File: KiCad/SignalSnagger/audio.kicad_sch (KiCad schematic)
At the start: 35 parts, among them J301 AudioJack4, U301 LM386, U302 LT6231

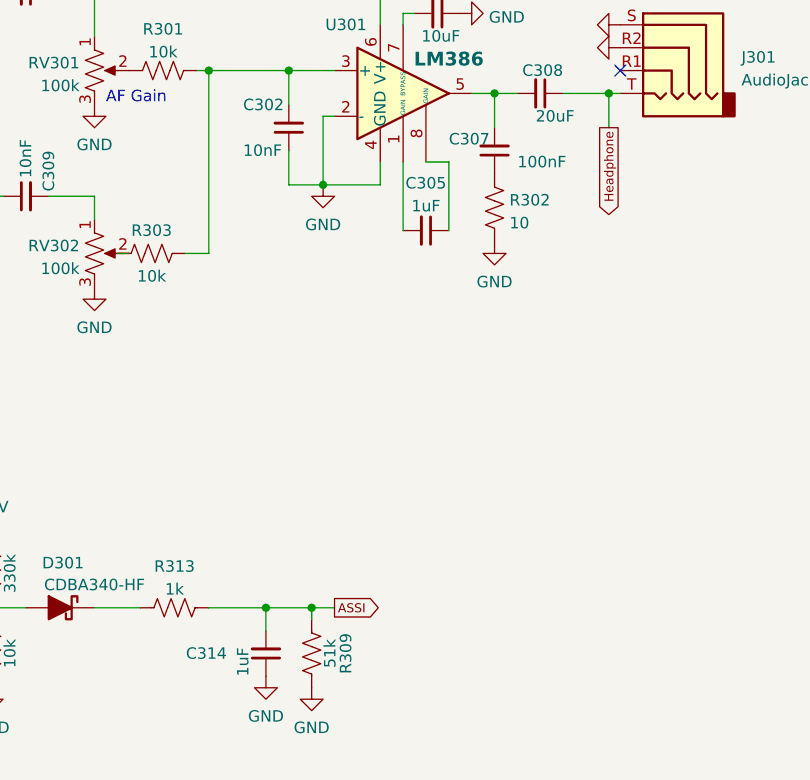
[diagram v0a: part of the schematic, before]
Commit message: Ver 0.22
o Schematic updates
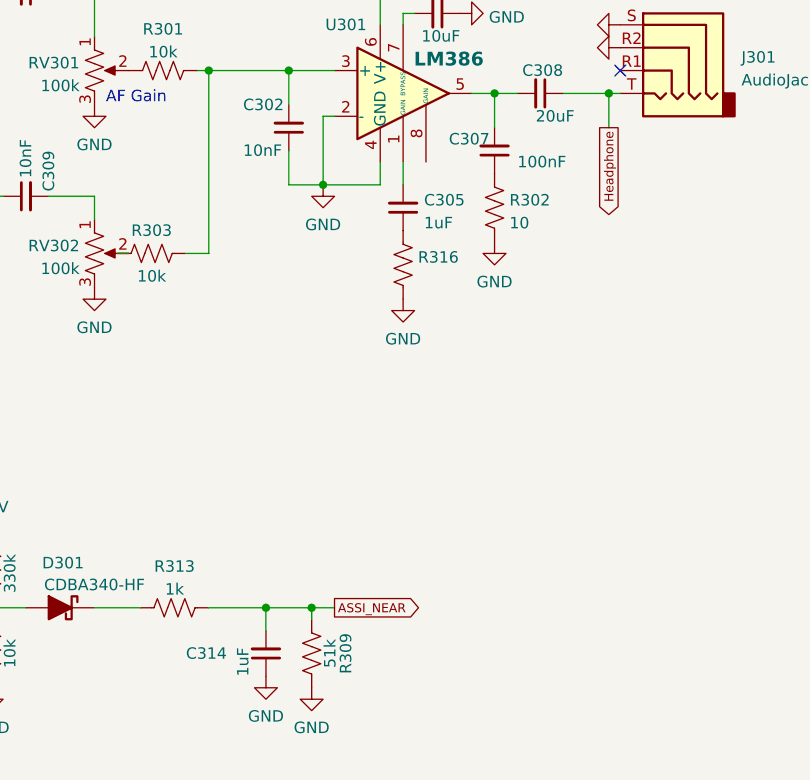
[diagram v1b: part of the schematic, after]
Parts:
- added R316: (no value), symbol Device:R_US
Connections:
- net GND: now also R316.2
- net at U301.8 (GAIN): no longer C305.1
- net ASSI renamed ASSI_NEAR
- new net: C305.1, R316.1
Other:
- moved on the sheet: C305
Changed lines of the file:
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@@
   (title_block
     (title "SignalSnagger")
-    (date "2023-12-19")
-    (rev "0.21")
+    (date "2024-02-01")
+    (rev "0.22")
   )
   (junction (at 66.04 128.27) (diameter 0) (color 0 0 0 0)
@@
     (stroke (width 0) (type default) (color 0 0 0 0))
   )
-  (wire (pts (xy 193.04 69.85) (xy 193.04 77.47))
+  (wire (pts (xy 193.04 69.85) (xy 193.04 72.39))
     (stroke (width 0) (type default) (color 0 0 0 0))
   )
@@
     (stroke (width 0) (type default) (color 0 0 0 0))
   )
-  (wire (pts (xy 198.12 77.47) (xy 198.12 69.85))
-    (stroke (width 0) (type default) (color 0 0 0 0))
-  )
   (wire (pts (xy 180.34 59.69) (xy 185.42 59.69))
     (stroke (width 0) (type default) (color 0 0 0 0))
@@
   )
   (wire (pts (xy 180.34 68.58) (xy 180.34 72.39))
-    (stroke (width 0) (type default) (color 0 0 0 0))
-  )
-  (wire (pts (xy 198.12 69.85) (xy 195.58 69.85))
     (stroke (width 0) (type default) (color 0 0 0 0))
   )
@@
     )
   )
-  (global_label "ASSI" (shape output) (at 185.42 119.38 0) (fields_autoplaced)
+  (global_label "ASSI_NEAR" (shape output) (at 185.42 119.38 0) (fields_autoplaced)
     (effects (font (size 1 1)) (justify left))
-    (property "Intersheet References" "${INTERSHEET_REFS}" (id 0) (at 190.5581 119.3175 0)
+    (property "Intersheet References" "${INTERSHEET_REFS}" (id 0) (at 195.1295 119.3175 0)
       (effects (font (size 1 1)) (justify left) hide)
     )
@@
     (pin "1")
   )
+  (symbol (lib_id "Device:R_US") (at 193.04 81.28 0) (unit 1)
+    (in_bom yes) (on_board yes) (fields_autoplaced)
+    (property "Reference" "R316" (id 0) (at 194.691 80.4453 0)
+      (effects (font (size 1.27 1.27)) (justify left))
+    )
+    (property "Value" "" (id 1) (at 194.691 82.9822 0)
+      (effects (font (size 1.27 1.27)) (justify left))
+    )
+    (property "Footprint" "" (id 2) (at 194.056 81.534 90)
+      (effects (font (size 1.27 1.27)) hide)
+    )
+    (property "Datasheet" "~" (id 3) (at 193.04 81.28 0)
+      (effects (font (size 1.27 1.27)) hide)
+    )
+    (pin "1")
+    (pin "2")
+  )
   (symbol (lib_id "Device:R_US") (at 78.74 116.84 90) (unit 1)
     (in_bom yes) (on_board yes)
@@
     (pin "1")
   )
-  (symbol (lib_id "Device:C_Small") (at 195.58 77.47 270) (unit 1)
-    (in_bom yes) (on_board yes) (fields_autoplaced)
-    (property "Reference" "C305" (id 0) (at 195.5736 72.2081 90))
-    (property "Value" "1uF" (id 1) (at 195.5736 74.745 90))
-    (property "Footprint" "" (id 2) (at 195.58 77.47 0)
-      (effects (font (size 1.27 1.27)) hide)
-    )
-    (property "Datasheet" "~" (id 3) (at 195.58 77.47 0)
+  (symbol (lib_id "Device:C_Small") (at 193.04 74.93 180) (unit 1)
+    (in_bom yes) (on_board yes) (fields_autoplaced)
+    (property "Reference" "C305" (id 0) (at 195.3641 74.0889 0)
+      (effects (font (size 1.27 1.27)) (justify right))
+    )
+    (property "Value" "1uF" (id 1) (at 195.3641 76.6258 0)
+      (effects (font (size 1.27 1.27)) (justify right))
+    )
+    (property "Footprint" "" (id 2) (at 193.04 74.93 0)
+      (effects (font (size 1.27 1.27)) hide)
+    )
+    (property "Datasheet" "~" (id 3) (at 193.04 74.93 0)
       (effects (font (size 1.27 1.27)) hide)
     )
@@
       (effects (font (size 1.27 1.27)) hide)
     )
+    (pin "1")
+  )
+  (symbol (lib_id "power:GND") (at 193.04 85.09 0) (unit 1)
+    (in_bom yes) (on_board yes) (fields_autoplaced)
+    (property "Reference" "#PWR0304" (id 0) (at 193.04 91.44 0)
+      (effects (font (size 1.27 1.27)) hide)
+    )
+    (property "Value" "GND" (id 1) (at 193.04 89.5334 0))
+    (property "Footprint" "" (id 2) (at 193.04 85.09 0)
+      (effects (font (size 1.27 1.27)) hide)
+    )
+    (property "Datasheet" "" (id 3) (at 193.04 85.09 0)
+      (effects (font (size 1.27 1.27)) hide)
+    )
